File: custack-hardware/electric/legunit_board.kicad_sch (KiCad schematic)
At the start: 26 parts, among them J10 Conn_01x03, J11 Conn_01x03, J12 Conn_01x03, J7 Conn_01x04, J8 Conn_01x03, J9 Conn_01x03, U2 20MHz 16KB FLASH, U3 MCP1702T-3302E/CB, U4 74LVC1G07, U5 74LVC1G07, U6 74LVC1G07, U7 74LVC1G07

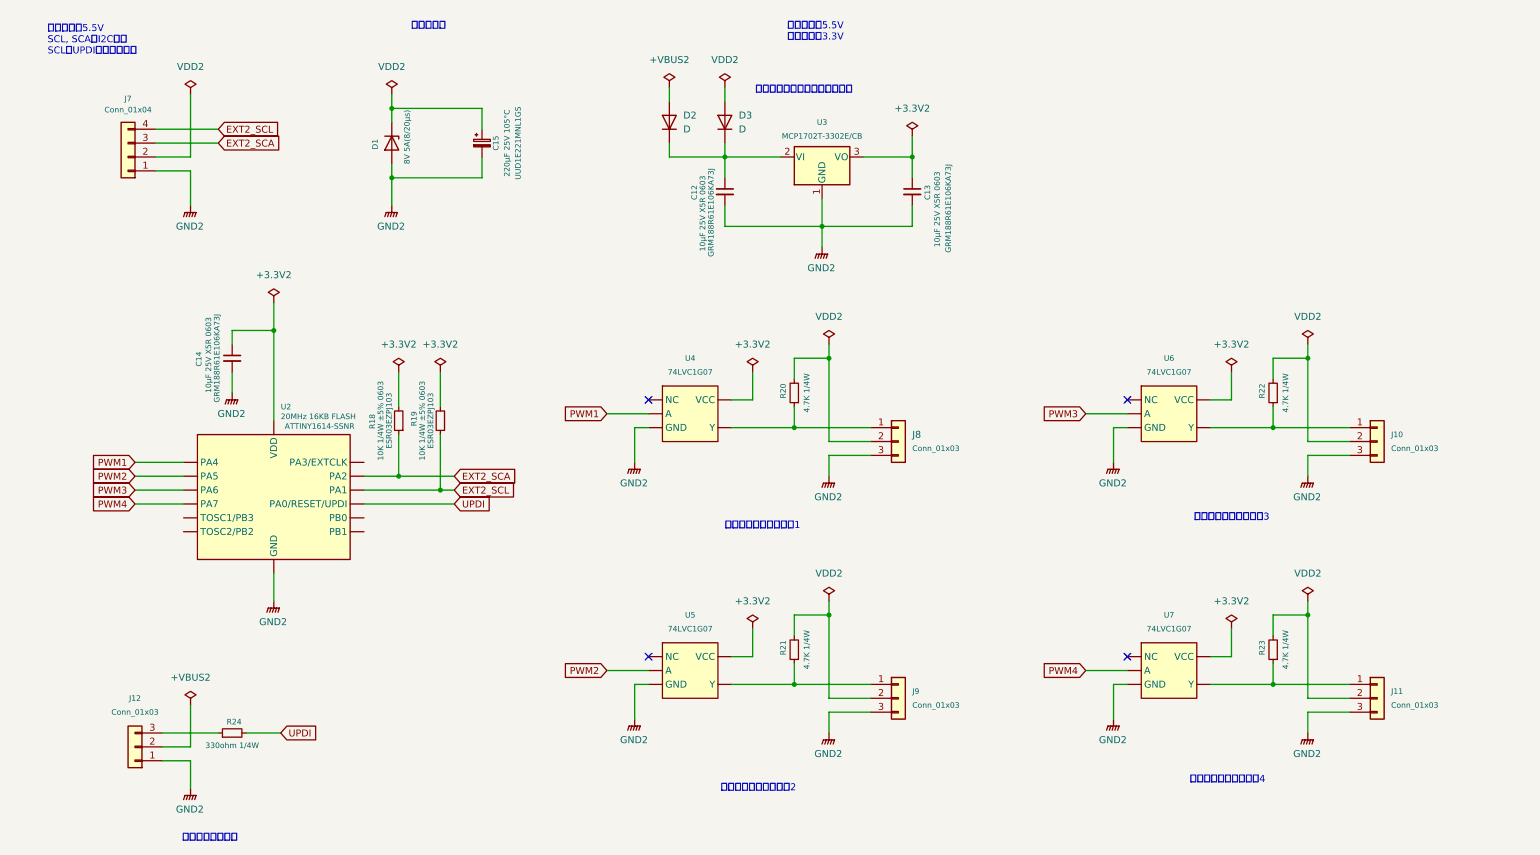
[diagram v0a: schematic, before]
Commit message: electric circut complete
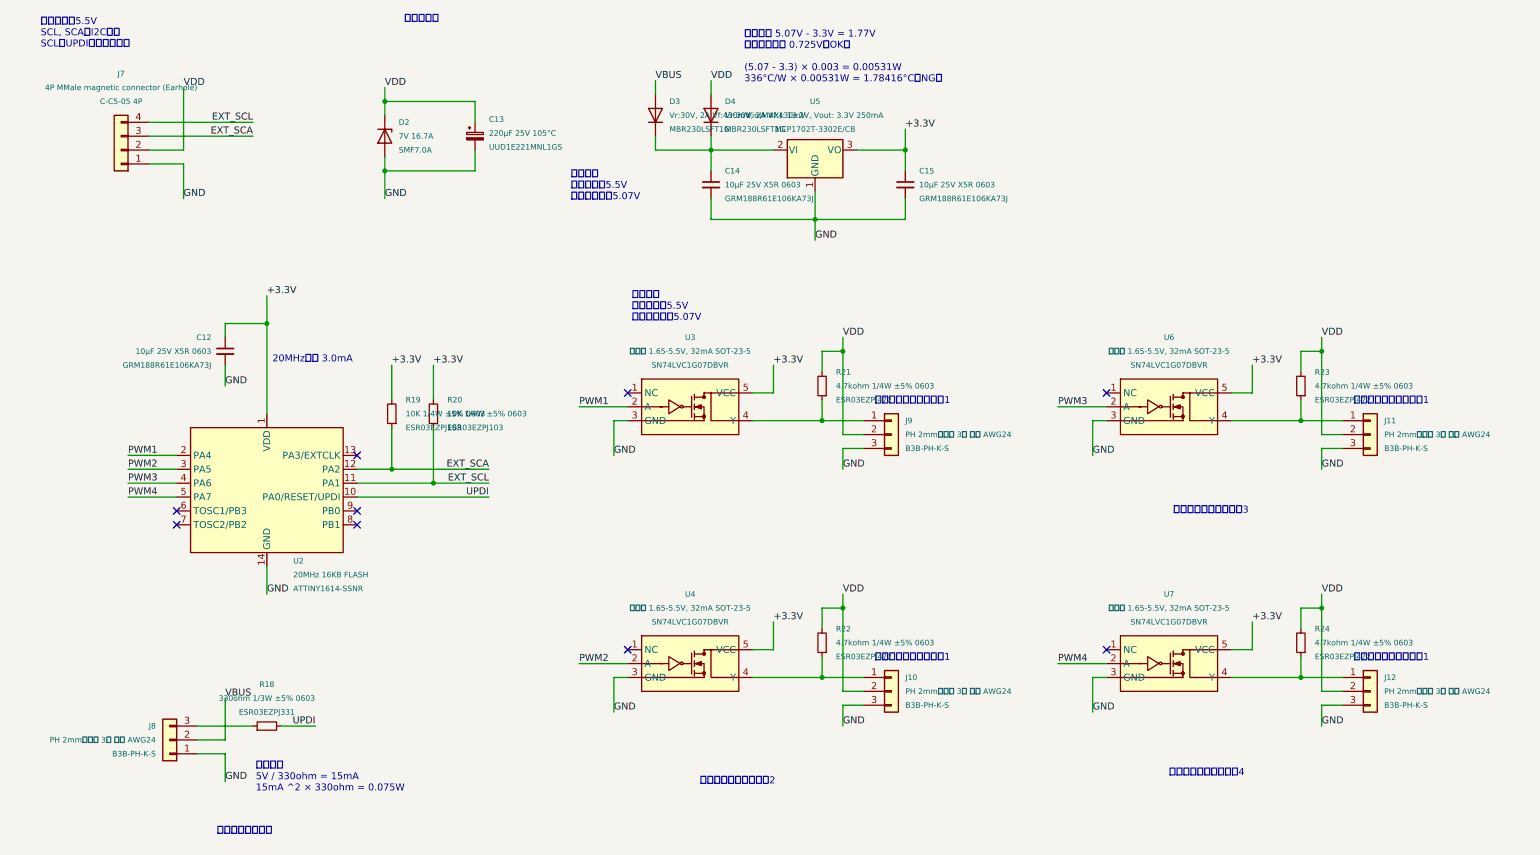
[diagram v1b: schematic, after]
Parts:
- removed C13: 10µF 25V X5R 0603, Capacitor_SMD:C_0603_1608Metric, symbol My_Device:C_Small
- removed C15: 220µF 25V 105°C, Capacitor_SMD:CP_Elec_8x10, symbol My_Device:C_Polarized_Small
- removed D1: 8V 5A(8/20µs), symbol My_Device:D_Zener
- removed D2: D, symbol My_Device:D
- removed U3: MCP1702T-3302E/CB, Package_TO_SOT_SMD:SOT-89-3, symbol Regulator_Linear:MCP1700x-120xxMB
- removed U4, U5, U6, U7: 74LVC1G07, symbol My_Device:74LVC1G07
- added C13: 220µF 25V 105°C, Capacitor_SMD:CP_Elec_8x10, symbol My_Device:C_Polarized_Small
- added C15: 10µF 25V X5R 0603, Capacitor_SMD:C_0603_1608Metric, symbol My_Device:C_Small
- added D2: 7V 16.7A, Diode_SMD:D_SOD-123F, symbol My_Device:D_Zener
- added D4: Vr:30V, 2A Vf:430mV, Diode_SMD:D_SOD-123F, symbol My_Device:D
- added U3, U4, U6, U7: 非反転 1.65-5.5V, 32mA SOT-23-5, Package_TO_SOT_SMD:SC-74A-5_1.55x2.9mm_P0.95mm, symbol My_Device:SN74LVC1G07DBVR
- added U5: Vin(MAX): 13.2V, Vout: 3.3V 250mA, Package_TO_SOT_SMD:SOT-23-3, symbol Regulator_Linear:MCP1700x-120xxMB
- D3: value D -> Vr:30V, 2A Vf:430mV; footprint (none) -> Diode_SMD:D_SOD-123F; 型式 (none) -> MBR230LSFT1G
- J10, J11, J12, J8, J9: value Conn_01x03 -> PH 2mmピッチ 3極 オス AWG24; footprint (none) -> Connector_JST:JST_PH_B3B-PH-K_1x03_P2.00mm_Vertical; 型式 (none) -> B3B-PH-K-S
- J7: value Conn_01x04 -> 4P MMale magnetic connector (Earhole); footprint (none) -> Connector_PinHeader_2.54mm:PinHeader_1x04_P2.54mm_Vertical; 型式 (none) -> C-C5-05 4P
- R18: value 10K 1/4W ±5% 0603 -> 330ohm 1/3W ±5% 0603; 型式 ESR03EZPJ103 -> ESR03EZPJ331
- R20: value 4.7K 1/4W -> 10K 1/4W ±5% 0603; footprint (none) -> Resistor_SMD:R_0603_1608Metric; 型式 (none) -> ESR03EZPJ103
- R21, R22, R23: value 4.7K 1/4W -> 4.7kohm 1/4W ±5% 0603; footprint (none) -> Resistor_SMD:R_0603_1608Metric; 型式 (none) -> ESR03EZPJ472
- R24: value 330ohm 1/4W -> 4.7kohm 1/4W ±5% 0603; footprint (none) -> Resistor_SMD:R_0603_1608Metric; 型式 (none) -> ESR03EZPJ472
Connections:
- net PWM1: now also U2.2 (PA4), U3.2 (A); no longer U2. (PB1)
- net PWM2: now also U2.3 (PA5), U4.2 (A); no longer U2. (PB1)
- net PWM3: now also U2.4 (PA6), U6.2 (A); no longer U2. (PB1)
- net PWM4: now also U2.5 (PA7), U7.2 (A); no longer U2. (PB1)
- net UPDI: now also R18.2, U2.10 (PA0/RESET/UPDI); no longer R24.2, U2. (PB1)
- net at J9.1 (Pin_1), R21.1: now also U3.4 (Y)
- net VDD: now reaches J7.2 (Pin_2)
- net VDD: now also J10.2 (Pin_2), J11.2 (Pin_2), J12.2 (Pin_2), J9.2 (Pin_2), R21.2, R22.2, R23.2, R24.2, C13.1, D2.1 (K), D4.2 (A)
- net at R24.1: now also J12.1 (Pin_1), U7.4 (Y); no longer J12.3 (Pin_3)
- net at D3.1 (K): now also C14.1, D4.1 (K), U5.2 (VI); no longer C12.1
- net at J11.1 (Pin_1), R23.1: now also U6.4 (Y)
- net EXT_SCL: now reaches R20.1
- net EXT_SCL: now also J7.4 (Pin_4), U2.11 (PA1); no longer J8.1 (Pin_1)
- net at J10.1 (Pin_1), R22.1: now also U4.4 (Y)
- net +3.3V: now reaches R19.2
- net +3.3V: now also C12.1, R20.2, U2.1 (VDD), C15.1, U3.5 (VCC), U4.5 (VCC), U5.3 (VO), U6.5 (VCC), U7.5 (VCC)
- net VBUS: now reaches J8.2 (Pin_2)
- net VBUS: now also D3.2 (A); no longer R20.2
- removed net EXT2_SCA: J7.3 (Pin_3), R18.1, U2. (PB1)
- removed net EXT2_SCL: J7.4 (Pin_4), R19.1, U2. (PB1)
- net GND2 renamed GND
- net GND: now also J12.3 (Pin_3), J8.1 (Pin_1), U2.14 (GND), C13.2, C15.2, D2.2 (A), U3.3 (GND), U4.3 (GND), U5.1 (GND), U6.3 (GND), U7.3 (GND); no longer J12.1 (Pin_1), J8.3 (Pin_3), U2. (PB1)
- new net: J8.3 (Pin_3), R18.1
- new net EXT_SCA: J7.3 (Pin_3), R19.1, U2.12 (PA2)
- no-connect marks 4 -> 9
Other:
- note added: "20MHz駆動 3.0mA"
- note added: "保護抵抗 5V / 330ohm = 15mA 15mA ^2 × 330ohm = 0.075W"
- note added: "入力電圧 5.07V - 3.3V = 1.77V ドロップ電圧 0.725V（OK） (5.07 - 3.3) × 0.003 = 0.00531W 336°C/W × 0.00531W = 1.78416°C（NG）"
- note added: "電圧降下 入力電圧：5.5V 降下後電圧：5.07V"
- note removed: "ショットキーバリアダイオード"
- note removed: "入力電圧：5.5V 出力電圧：3.3V"
